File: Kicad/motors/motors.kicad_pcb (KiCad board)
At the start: 2 copper layers, 80 x 100 mm, 64 parts, among them IC101 TLV1117-50, IC201 PIC16F1778-IP, IC301 MCP2221A-ISL, K101 Battery, K201 MCU 1, K202 MCU 2, K203 ICSP, K301 FRONT, K302 MICRO USB B, K303 M20-782084x, K304 M20-782084x, K305 SERVO LEFT, K306 SERVO RIGHT, T101 DMP2305U, T102 DMP2305U

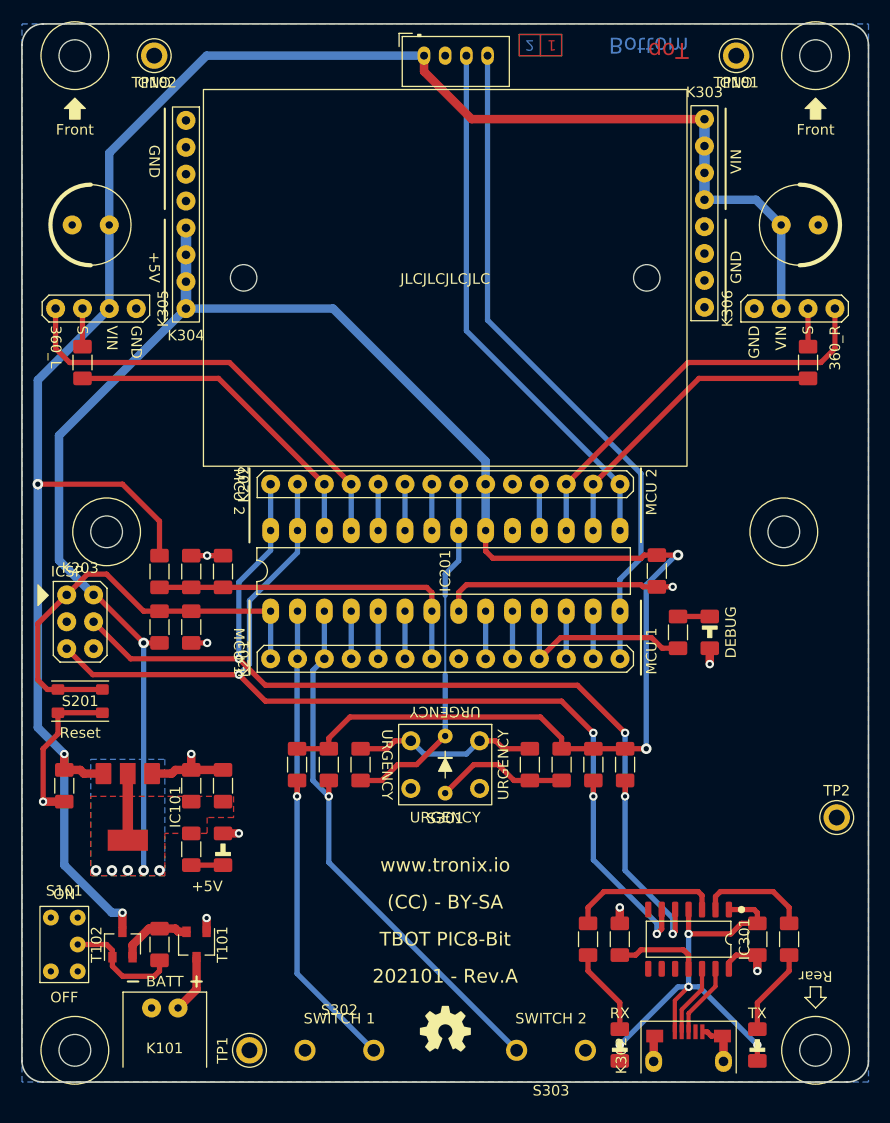
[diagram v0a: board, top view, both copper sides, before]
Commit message: Update Motor
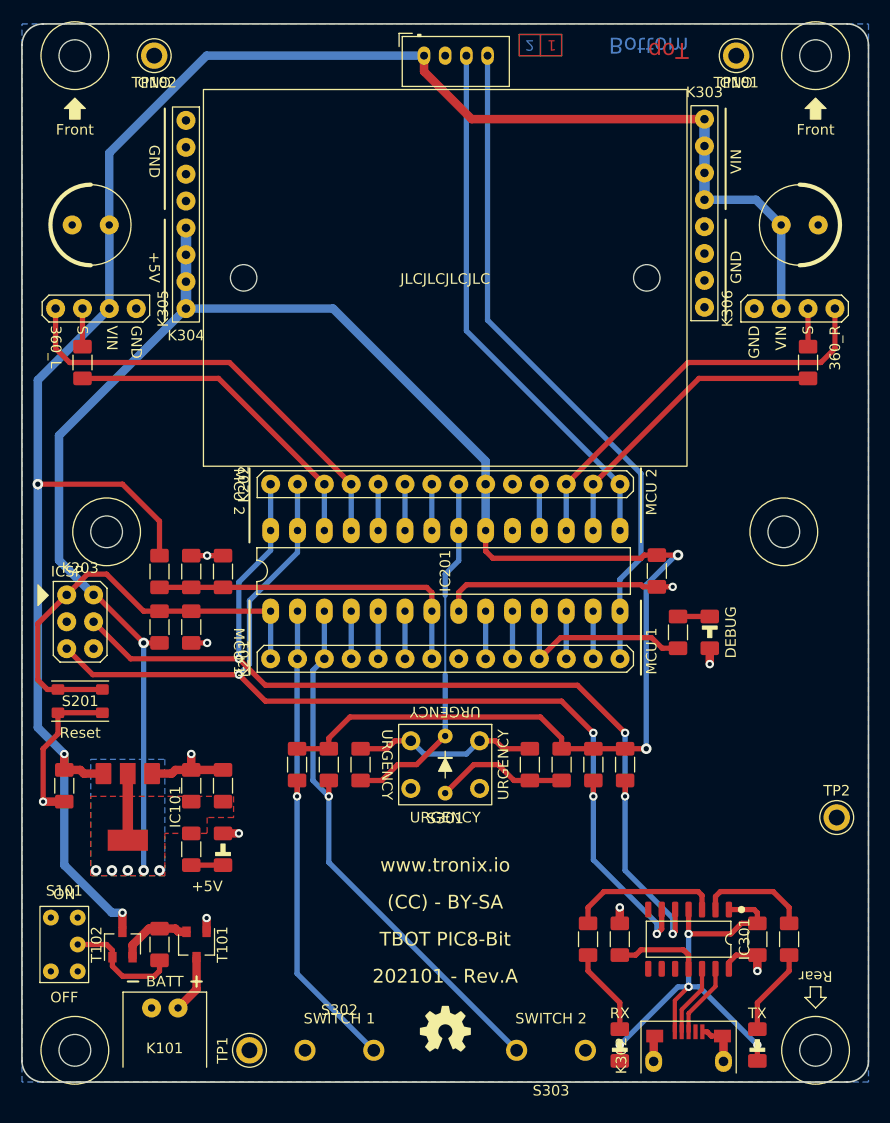
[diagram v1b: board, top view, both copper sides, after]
